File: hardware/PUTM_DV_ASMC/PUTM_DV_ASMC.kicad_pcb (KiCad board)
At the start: 4 copper layers, 84.6 x 88.2 mm, 180 parts, among them IC1 BTS722204ESAXUMA1, IC2 BTS722204ESAXUMA1, J1 FTSH-107-01-L-D-K, J2 IPBS-110-01-XX-D-GP, J4 74650073R, J5 74650073R, K2 FINDER-32.21-x000, Q1 30V/5A, Q2 BUK6D210, Q3 BUK6D210, Q6 BSS138, T1 TP_VCC, T2 TP_+5V, T3 TP_+3V3, T6 TP_VCC, T8 TP_+5V, U1 LM4040C33FTA, U14 FODM217B, U15 FODM217B, U2 STM32G484RETx, U3 LM1117-3.3, U4 TPS54202HDDCR, U5 ADM3057ExRW, U6 ADM3057ExRW, U7 74AHCT1G125, Y1 ATX-11-F-32.000MHZ-F05-T

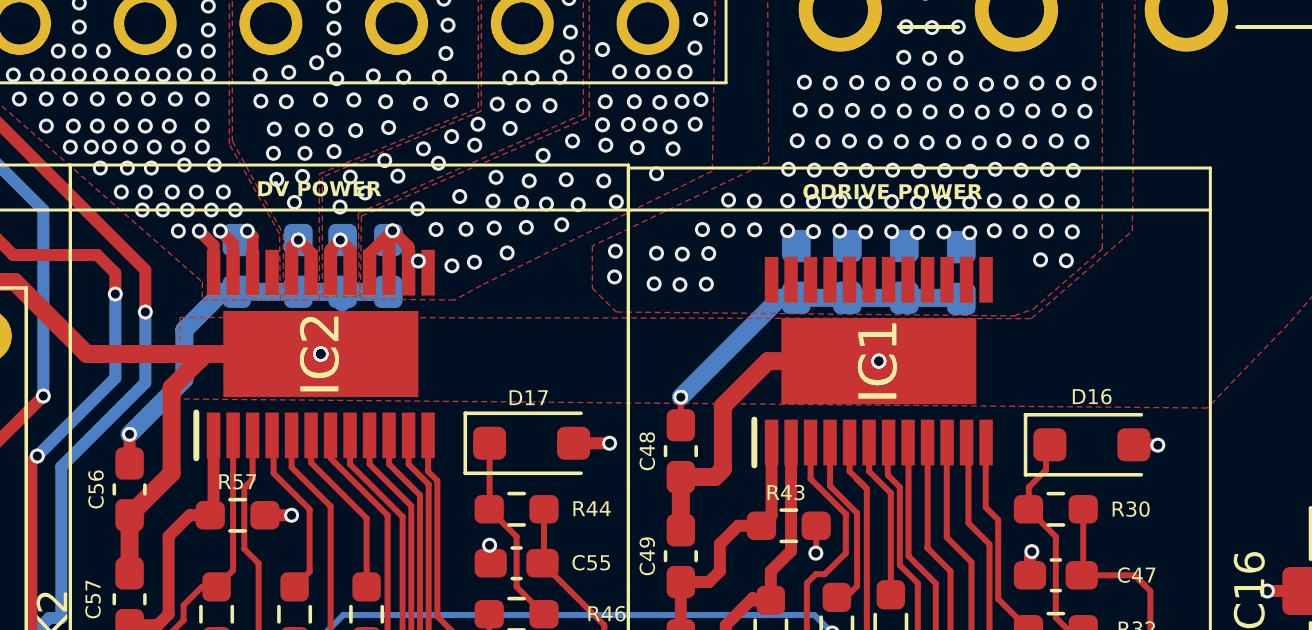
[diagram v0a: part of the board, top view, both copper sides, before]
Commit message: update pcb layout4 - before review
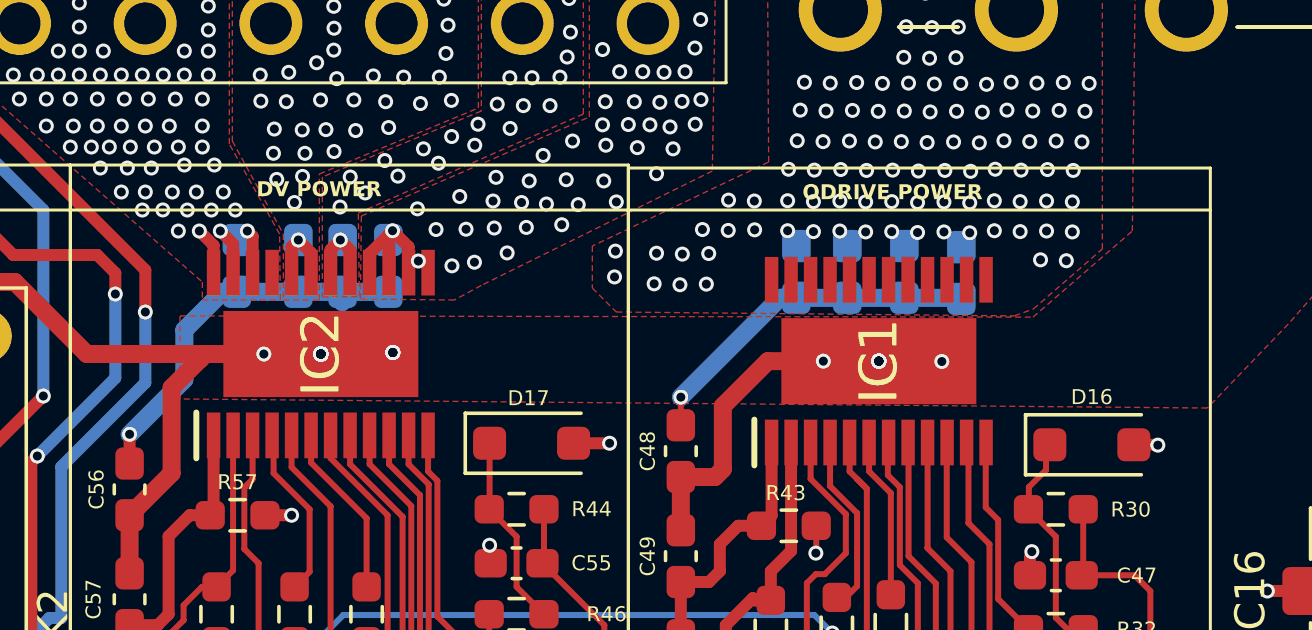
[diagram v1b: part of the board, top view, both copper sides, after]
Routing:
- net +BATT: track 42.6 -> 44.7 mm, vias 11 -> 37
